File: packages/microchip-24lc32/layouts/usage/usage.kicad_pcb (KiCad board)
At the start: 2 copper layers, 4 parts

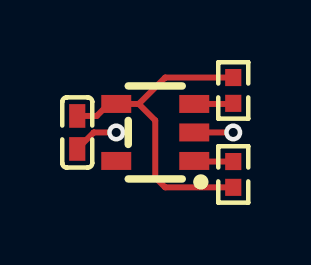
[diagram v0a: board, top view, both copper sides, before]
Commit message: many packages building
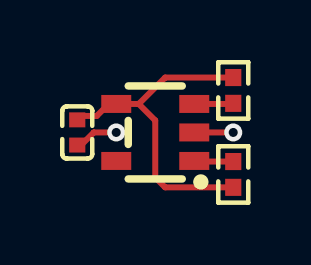
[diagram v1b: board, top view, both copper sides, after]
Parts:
- C1: value 100nF ±10% 16V X7R -> 1.0000000000000001e-07F
- R1, R2: value 10kΩ ±1% 62.5mW -> 10000.0Ω
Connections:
- net GND renamed lv
- net VCC renamed eeprom-power-hv-0

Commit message: review tool updates
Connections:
- net eeprom-power-hv-0 renamed hv
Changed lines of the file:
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@@
 			(usegerberadvancedattributes yes)
 			(creategerberjobfile yes)
-			(dashed_line_dash_ratio 12.000000)
-			(dashed_line_gap_ratio 3.000000)
+			(dashed_line_dash_ratio 12)
+			(dashed_line_gap_ratio 3)
 			(svgprecision 4)
 			(plotframeref no)
@@
 			(hpglpennumber 1)
 			(hpglpenspeed 20)
-			(hpglpendiameter 15.000000)
+			(hpglpendiameter 15)
 			(pdf_front_fp_property_popups yes)
 			(pdf_back_fp_property_popups yes)
@@
 	(net 0 "")
 	(net 1 "lv")
-	(net 2 "eeprom-power-hv-0")
+	(net 2 "hv")
 	(net 3 "SDA")
 	(net 4 "WP")
@@
 			(size 0.57 0.54)
 			(layers "F.Cu" "F.Paste" "F.Mask")
-			(net 2 "eeprom-power-hv-0")
+			(net 2 "hv")
 		)
 		(pad "1" smd rect
@@
 			(size 0.57 0.54)
 			(layers "F.Cu" "F.Paste" "F.Mask")
-			(net 2 "eeprom-power-hv-0")
+			(net 2 "hv")
 		)
 		(pad "1" smd rect
@@
 			(size 0.5 0.54)
 			(layers "F.Cu" "F.Paste" "F.Mask")
-			(net 2 "eeprom-power-hv-0")
+			(net 2 "hv")
 		)
 		(embedded_fonts no)
@@
 			(size 1 0.6)
 			(layers "F.Cu" "F.Mask" "F.Paste")
-			(net 2 "eeprom-power-hv-0")
+			(net 2 "hv")
 		)
 		(pad "5" smd rect
